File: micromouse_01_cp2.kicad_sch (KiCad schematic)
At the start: 36 parts, among them IC2 MPU-6500, IC5 DRV8835DSSR, M1 MK06-4.5, M2 MK06-4.5, U10 MA730, U11 MA730, U13 MCP3464T-E/NC, U9 ESP32-S3-PICO-1-N8R2

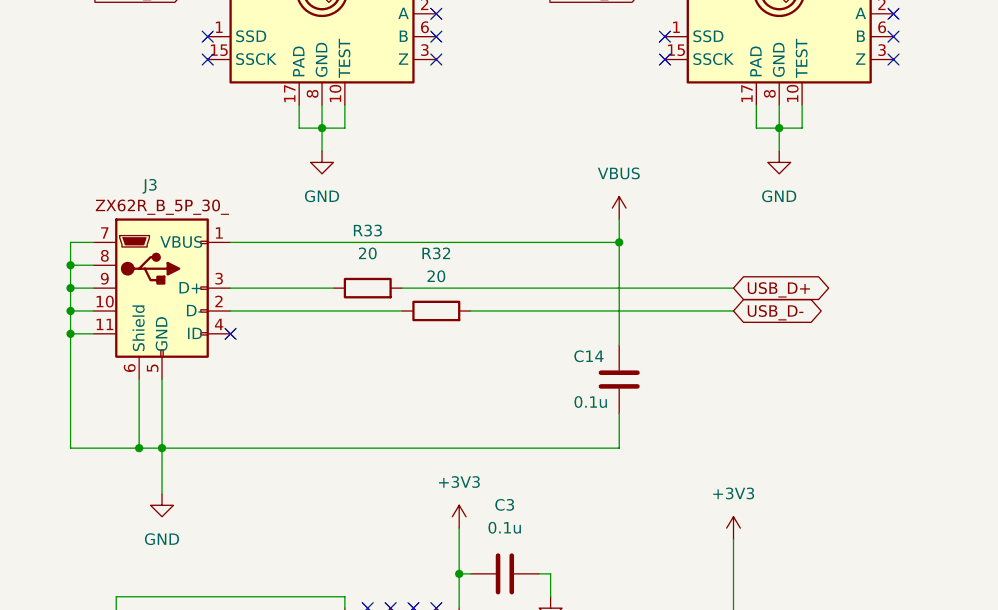
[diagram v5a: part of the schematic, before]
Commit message: [update]いい感じ
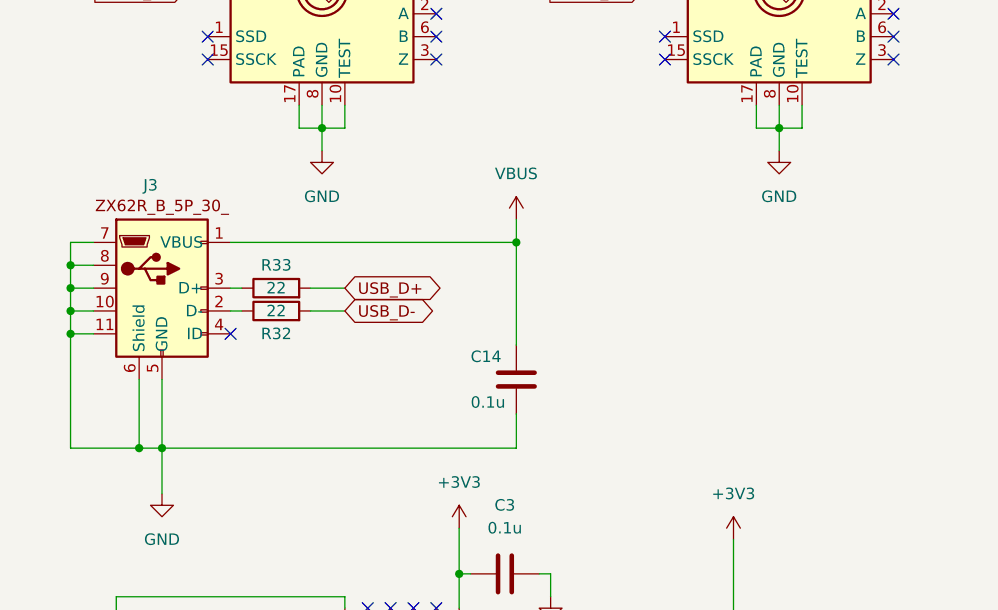
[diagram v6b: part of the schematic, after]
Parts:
- R32, R33: value 20 -> 22
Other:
- moved on the sheet: C14, R32, R33
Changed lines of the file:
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@@
   (junction (at 243.84 129.54) (diameter 0) (color 0 0 0 0)
   )
-  (junction (at 91.44 66.04) (diameter 0) (color 0 0 0 0)
+  (junction (at 80.01 66.04) (diameter 0) (color 0 0 0 0)
   )
   (junction (at 175.26 17.78) (diameter 0) (color 0 0 0 0)
@@
     (stroke (width 0) (type default))
   )
-  (wire (pts (xy 67.31 71.12) (xy 104.14 71.12))
+  (wire (pts (xy 57.15 71.12) (xy 60.96 71.12))
     (stroke (width 0) (type default))
   )
@@
     (stroke (width 0) (type default))
   )
-  (wire (pts (xy 48.26 66.04) (xy 91.44 66.04))
+  (wire (pts (xy 48.26 66.04) (xy 80.01 66.04))
     (stroke (width 0) (type default))
   )
@@
     (stroke (width 0) (type default))
   )
-  (wire (pts (xy 74.93 73.66) (xy 104.14 73.66))
+  (wire (pts (xy 57.15 73.66) (xy 60.96 73.66))
     (stroke (width 0) (type default))
   )
@@
     (stroke (width 0) (type default))
   )
-  (wire (pts (xy 48.26 71.12) (xy 59.69 71.12))
+  (wire (pts (xy 48.26 71.12) (xy 49.53 71.12))
     (stroke (width 0) (type default))
   )
@@
     (stroke (width 0) (type default))
   )
-  (wire (pts (xy 40.64 88.9) (xy 91.44 88.9))
+  (wire (pts (xy 40.64 88.9) (xy 80.01 88.9))
     (stroke (width 0) (type default))
   )
@@
     (stroke (width 0) (type default))
   )
-  (wire (pts (xy 91.44 66.04) (xy 91.44 63.5))
+  (wire (pts (xy 80.01 66.04) (xy 80.01 63.5))
     (stroke (width 0) (type default))
   )
@@
     (stroke (width 0) (type default))
   )
-  (wire (pts (xy 91.44 85.09) (xy 91.44 88.9))
+  (wire (pts (xy 80.01 85.09) (xy 80.01 88.9))
     (stroke (width 0) (type default))
   )
@@
     (stroke (width 0) (type default))
   )
-  (wire (pts (xy 48.26 73.66) (xy 67.31 73.66))
+  (wire (pts (xy 48.26 73.66) (xy 49.53 73.66))
     (stroke (width 0) (type default))
   )
@@
     (stroke (width 0) (type default))
   )
-  (wire (pts (xy 91.44 77.47) (xy 91.44 66.04))
+  (wire (pts (xy 80.01 77.47) (xy 80.01 66.04))
     (stroke (width 0) (type default))
   )
@@
     )
   )
-  (global_label "USB_D-" (shape bidirectional) (at 104.14 73.66 0) (fields_autoplaced)
+  (global_label "USB_D-" (shape bidirectional) (at 60.96 73.66 0) (fields_autoplaced)
     (effects (font (size 1.27 1.27)) (justify left))
-    (property "Intersheetrefs" "${INTERSHEET_REFS}" (at 115.8565 73.66 0)
+    (property "Intersheetrefs" "${INTERSHEET_REFS}" (at 72.6765 73.66 0)
       (effects (font (size 1.27 1.27)) (justify left) hide)
     )
@@
     )
   )
-  (global_label "USB_D+" (shape bidirectional) (at 104.14 71.12 0) (fields_autoplaced)
+  (global_label "USB_D+" (shape bidirectional) (at 60.96 71.12 0) (fields_autoplaced)
     (effects (font (size 1.27 1.27)) (justify left))
-    (property "Intersheetrefs" "${INTERSHEET_REFS}" (at 115.8565 71.12 0)
+    (property "Intersheetrefs" "${INTERSHEET_REFS}" (at 72.6765 71.12 0)
       (effects (font (size 1.27 1.27)) (justify left) hide)
     )
@@
     )
   )
-  (symbol (lib_id "Device:R") (at 71.12 73.66 90) (unit 1)
-    (in_bom yes) (on_board yes) (dnp no) (fields_autoplaced)
-    (property "Reference" "R32" (at 71.12 67.31 90)
-      (effects (font (size 1.27 1.27)))
-    )
-    (property "Value" "20" (at 71.12 69.85 90)
-      (effects (font (size 1.27 1.27)))
-    )
-    (property "Footprint" "Resistor_SMD:R_0402_1005Metric" (at 71.12 75.438 90)
-      (effects (font (size 1.27 1.27)) hide)
-    )
-    (property "Datasheet" "~" (at 71.12 73.66 0)
+  (symbol (lib_id "Device:R") (at 53.34 73.66 90) (unit 1)
+    (in_bom yes) (on_board yes) (dnp no)
+    (property "Reference" "R32" (at 53.34 76.2 90)
+      (effects (font (size 1.27 1.27)))
+    )
+    (property "Value" "22" (at 53.34 73.66 90)
+      (effects (font (size 1.27 1.27)))
+    )
+    (property "Footprint" "Resistor_SMD:R_0402_1005Metric" (at 53.34 75.438 90)
+      (effects (font (size 1.27 1.27)) hide)
+    )
+    (property "Datasheet" "~" (at 53.34 73.66 0)
       (effects (font (size 1.27 1.27)) hide)
     )
@@
     )
   )
-  (symbol (lib_id "Device:R") (at 63.5 71.12 90) (unit 1)
-    (in_bom yes) (on_board yes) (dnp no) (fields_autoplaced)
-    (property "Reference" "R33" (at 63.5 64.77 90)
-      (effects (font (size 1.27 1.27)))
-    )
-    (property "Value" "20" (at 63.5 67.31 90)
-      (effects (font (size 1.27 1.27)))
-    )
-    (property "Footprint" "Resistor_SMD:R_0402_1005Metric" (at 63.5 72.898 90)
-      (effects (font (size 1.27 1.27)) hide)
-    )
-    (property "Datasheet" "~" (at 63.5 71.12 0)
+  (symbol (lib_id "Device:R") (at 53.34 71.12 90) (unit 1)
+    (in_bom yes) (on_board yes) (dnp no)
+    (property "Reference" "R33" (at 53.34 68.58 90)
+      (effects (font (size 1.27 1.27)))
+    )
+    (property "Value" "22" (at 53.34 71.12 90)
+      (effects (font (size 1.27 1.27)))
+    )
+    (property "Footprint" "Resistor_SMD:R_0402_1005Metric" (at 53.34 72.898 90)
+      (effects (font (size 1.27 1.27)) hide)
+    )
+    (property "Datasheet" "~" (at 53.34 71.12 0)
       (effects (font (size 1.27 1.27)) hide)
     )
@@
     )
   )
-  (symbol (lib_id "Device:C") (at 91.44 81.28 0) (unit 1)
+  (symbol (lib_id "Device:C") (at 80.01 81.28 0) (unit 1)
     (in_bom yes) (on_board yes) (dnp no)
-    (property "Reference" "C14" (at 86.36 78.74 0)
-      (effects (font (size 1.27 1.27)) (justify left))
-    )
-    (property "Value" "0.1u" (at 86.36 83.82 0)
-      (effects (font (size 1.27 1.27)) (justify left))
-    )
-    (property "Footprint" "Capacitor_SMD:C_0402_1005Metric" (at 92.4052 85.09 0)
-      (effects (font (size 1.27 1.27)) hide)
-    )
-    (property "Datasheet" "~" (at 91.44 81.28 0)
+    (property "Reference" "C14" (at 74.93 78.74 0)
+      (effects (font (size 1.27 1.27)) (justify left))
+    )
+    (property "Value" "0.1u" (at 74.93 83.82 0)
+      (effects (font (size 1.27 1.27)) (justify left))
+    )
+    (property "Footprint" "Capacitor_SMD:C_0402_1005Metric" (at 80.9752 85.09 0)
+      (effects (font (size 1.27 1.27)) hide)
+    )
+    (property "Datasheet" "~" (at 80.01 81.28 0)
       (effects (font (size 1.27 1.27)) hide)
     )
@@
     )
   )
-  (symbol (lib_id "power:VBUS") (at 91.44 63.5 0) (unit 1)
-    (in_bom yes) (on_board yes) (dnp no) (fields_autoplaced)
-    (property "Reference" "#PWR018" (at 91.44 67.31 0)
-      (effects (font (size 1.27 1.27)) hide)
-    )
-    (property "Value" "VBUS" (at 91.44 58.42 0)
-      (effects (font (size 1.27 1.27)))
-    )
-    (property "Footprint" "" (at 91.44 63.5 0)
-      (effects (font (size 1.27 1.27)) hide)
-    )
-    (property "Datasheet" "" (at 91.44 63.5 0)
-      (effects (font (size 1.27 1.27)) hide)
-    )
+  (symbol (lib_id "power:VBUS") (at 80.01 63.5 0) (unit 1)
+    (in_bom yes) (on_board yes) (dnp no) (fields_autoplaced)
+    (property "Reference" "#PWR018" (at 80.01 67.31 0)
+      (effects (font (size 1.27 1.27)) hide)
+    )
+    (property "Value" "VBUS" (at 80.01 58.42 0)
+      (effects (font (size 1.27 1.27)))
+    )
+    (property "Footprint" "" (at 80.01 63.5 0)
+      (effects (font (size 1.27 1.27)) hide)
+    )
+    (property "Datasheet" "" (at 80.01 63.5 0)
+      (effects (font (size 1.27 1.27)) hide)
+    )
